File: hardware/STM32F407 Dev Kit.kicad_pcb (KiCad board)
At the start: 4 copper layers, 65.2 x 58.4 mm, 153 parts, among them J1 GMSB0531112YEU, J10 Conn_01x04, J11 TBC 2.54mm 10A, J12 IMP34DT05, J2 Conn_01x06, J3 RJMG1S8008101BR, J4 B2B-XH-A(LF)(SN), J5 Conn_01x04, J7 SJ-3524-SMT, J8 GMSB0531112YEU, J9 Conn_01x04, SW1 SW TACT-SPST, SW2 SW TACT-SPST, SW3 SW TACT-SPST, U1 STM32F103CBT6, U2 DP83826IRHBR, U3 DRV8701ERGET, U4 DMHT6016LFJ-13, U5 ADS122C04IPW, U6 CS43L22, U7 STM32F407VGT6, U8 AP63203WU, U9 XC6206P182MR, Y1 ABM8G-8.000MHZ-18-D2Y-T, Y2 ABM8G-25.000MHZ-9-B4Y-T, Y3 ABM8G-8.000MHZ-18-D2Y-T

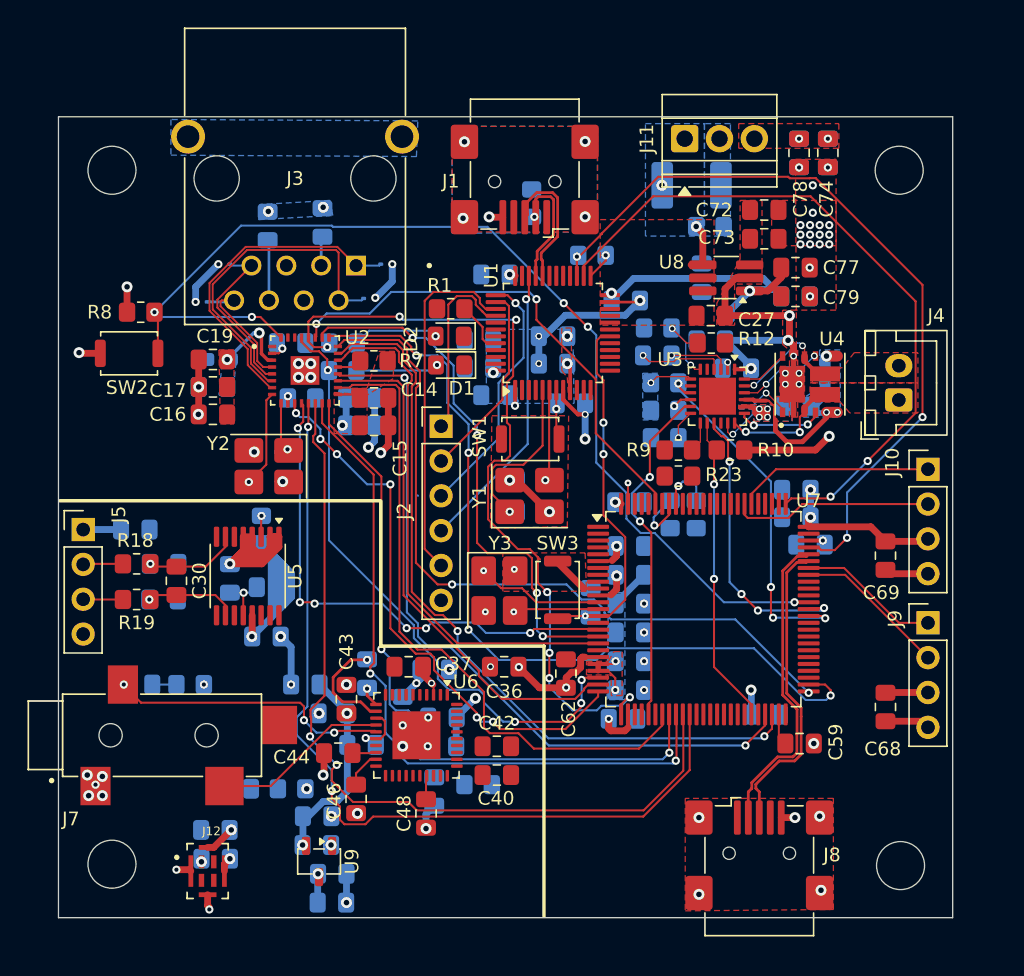
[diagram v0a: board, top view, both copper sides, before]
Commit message: Fix DRC errors
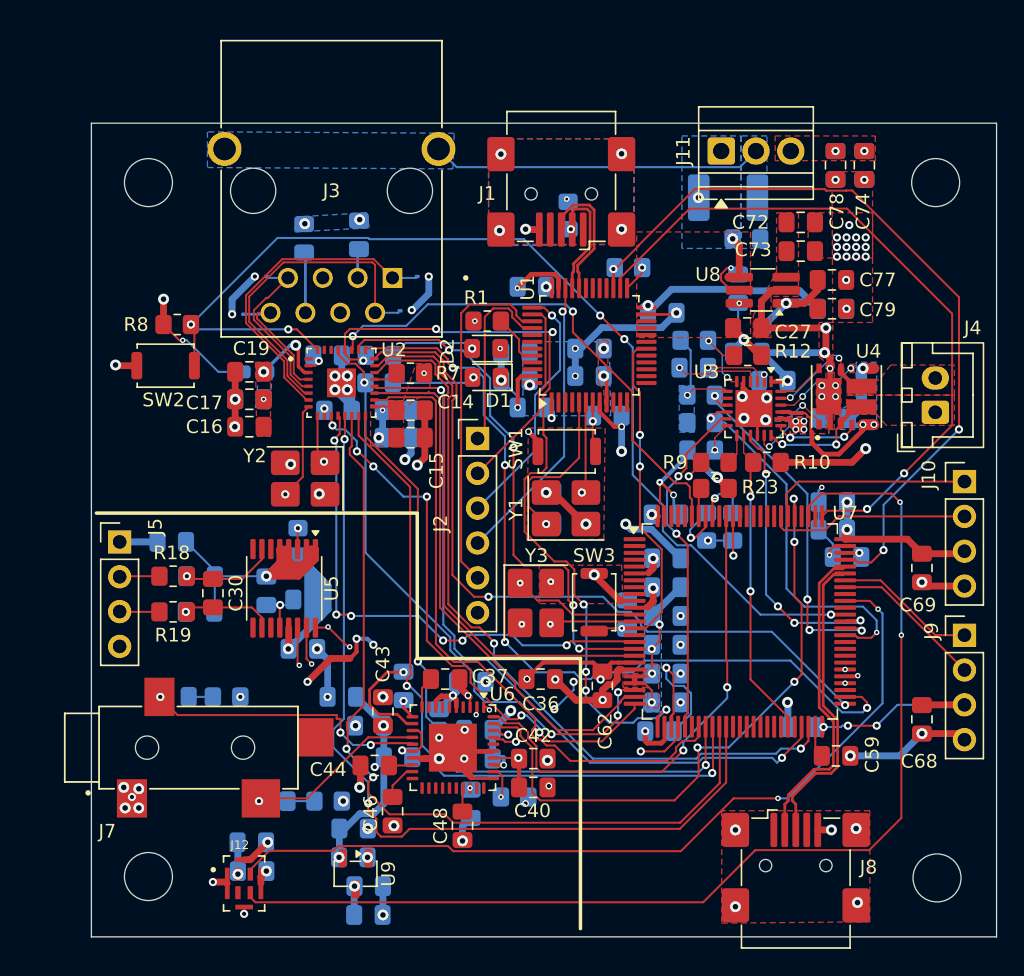
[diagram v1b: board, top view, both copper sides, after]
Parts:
- moved C12 2.81 mm to (174.7, 71.4)
- moved C13 2.81 mm to (174.7, 73.4)
- moved C14 2.81 mm to (175.7, 71.4)
- moved C15 2.81 mm to (175.7, 73.4)
- moved C32 2.81 mm to (160.4, 83.5)
- moved C46 2.81 mm to (174.4, 100.6)
- moved C56 2.81 mm to (194.3, 79.0)
- moved C70 2.81 mm to (184.9, 83.9)
- moved D4 2.81 mm to (175.3, 64.2)
- moved D6 2.81 mm to (163.1, 64.4)
- moved R18 2.81 mm to (158.4, 83.5)
- moved R9 2.81 mm to (197.9, 75.2)
- moved D3 2.81 mm to (176.6, 61.6)
- moved C16 2.81 mm to (163.9, 72.6)
- moved C17 2.81 mm to (163.9, 70.6)
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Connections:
- R24 pad 2: /[8] - STM32F407/SCL -> SCL
- R25 pad 1: /[8] - STM32F407/SDA -> SDA
- U7 pad 92: /[8] - STM32F407/SCL -> SCL
- U7 pad 93: /[8] - STM32F407/SDA -> SDA
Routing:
- net GND: track 135.0 -> 226.1 mm, vias 99 -> 119
- net MIC_CLK: track 0.00 -> 81.6 mm, vias 0 -> 2
- net +3V3: track 94.1 -> 162.2 mm, vias 20 -> 36
- net SDA: track 0.00 -> 66.0 mm, vias 0 -> 3
- net MIC_DOUT: track 0.00 -> 61.4 mm, vias 0 -> 2
- net ADC_RST: track 1.54 -> 54.0 mm, vias 1 -> 2
- net SCL: track 0.00 -> 51.2 mm, vias 0 -> 4
- net ADC_DRDY: track 0.00 -> 47.4 mm, vias 0 -> 2
- net CS43L22_SDIN: track 0.00 -> 46.8 mm, vias 0 -> 4
- net CS43L22_LRCK: track 0.00 -> 35.7 mm, vias 0 -> 2
- net CS43L22_RST: track 0.00 -> 30.9 mm, vias 0 -> 2
- net CS43L22_SCLK: track 0.00 -> 26.3 mm, vias 0 -> 4
- net SNSOUT: track 1.81 -> 27.5 mm, vias 1 -> 2
- net SHEILD: track 0.00 -> 24.2 mm
- net +1V8: track 14.8 -> 30.5 mm, vias 2 -> 4
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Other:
- board size 65.2 x 58.4 mm -> 66 x 59.3 mm
